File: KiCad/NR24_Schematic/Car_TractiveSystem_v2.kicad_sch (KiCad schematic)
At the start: 11 parts, among them J1 M_con, J2 F_con, K2 Key Switch Relay, M1 Zero_7R_Motor, SW3 100V E-stop (Right), SW4 100V E-stop (Left), U1 Sevcon_Gen4_Size6, U2 Throttle

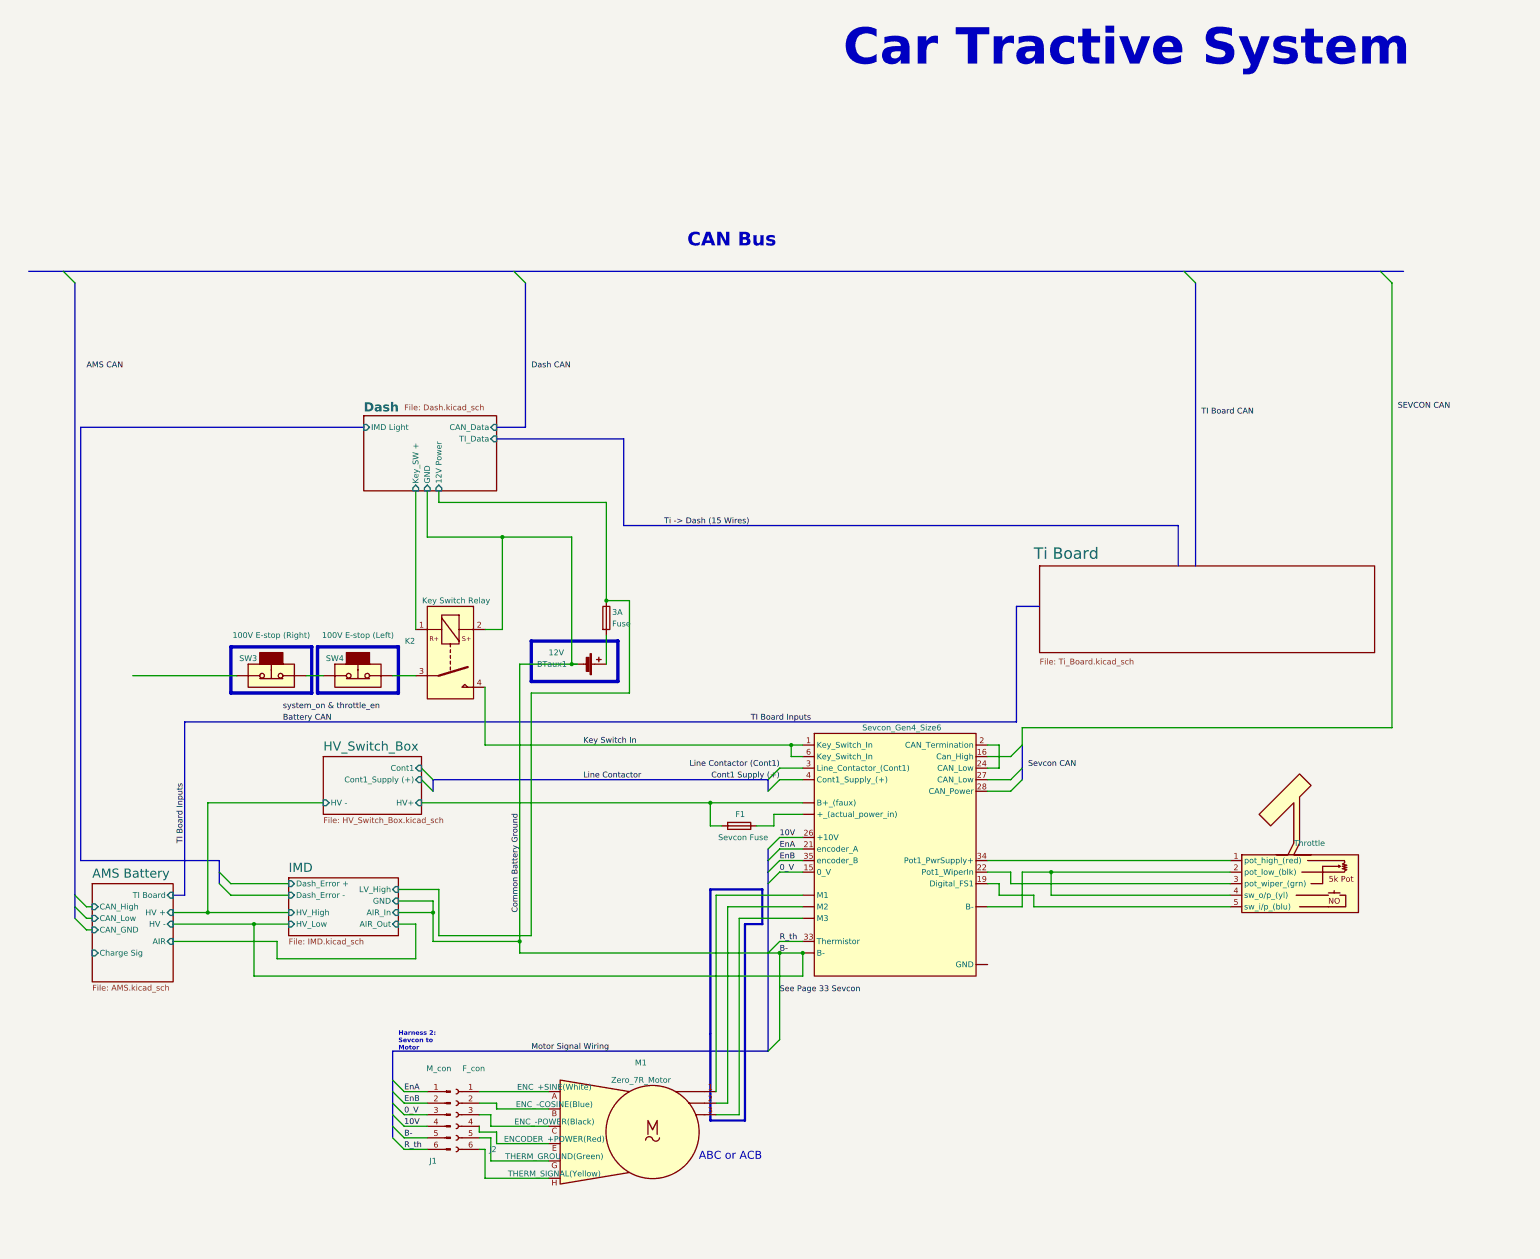
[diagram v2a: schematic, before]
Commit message: Updates
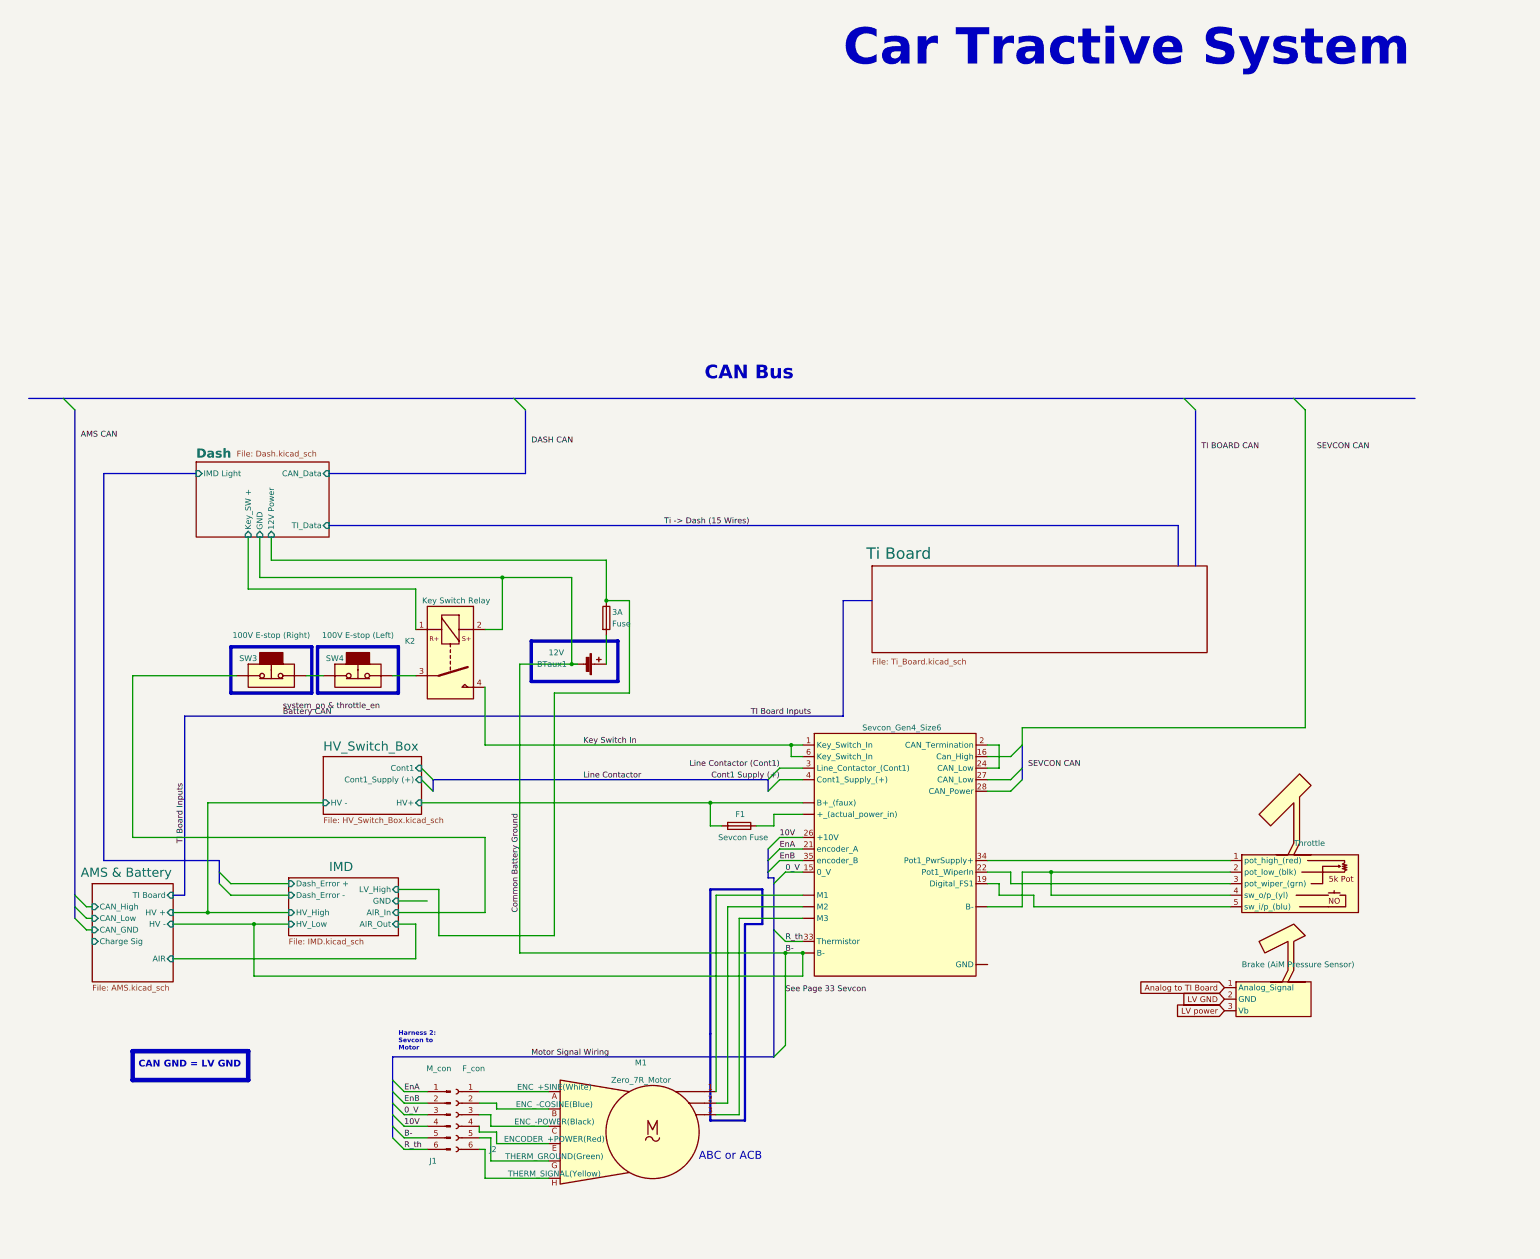
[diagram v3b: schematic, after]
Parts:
- added U7: Brake (AiM Pressure Sensor), symbol CamachosSymbols:Throttle
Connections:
- net IMD/AIR_In: now reaches SW3.1 (A)
- new net  LV power: U7.3 (Vb)
- new net Analog to TI Board: U7.1 (Analog_Signal)
- new net LV GND: U7.2 (GND)
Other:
- sheet AMS Battery renamed AMS & Battery
- note added: "CAN GND = LV GND"

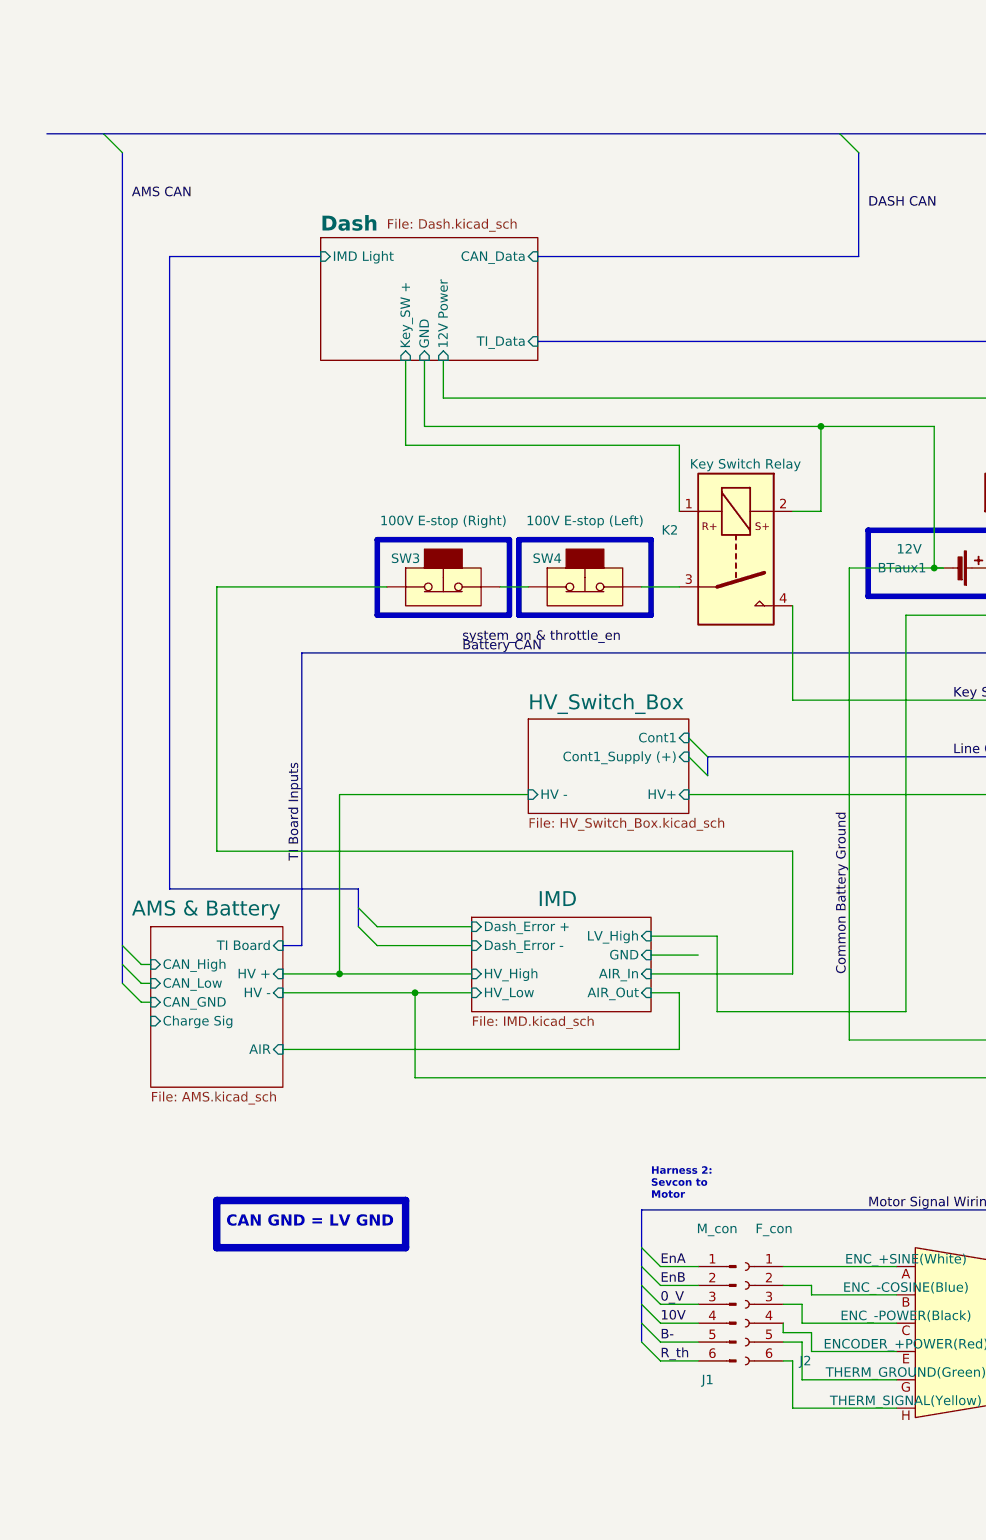
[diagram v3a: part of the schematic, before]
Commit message: Root Update
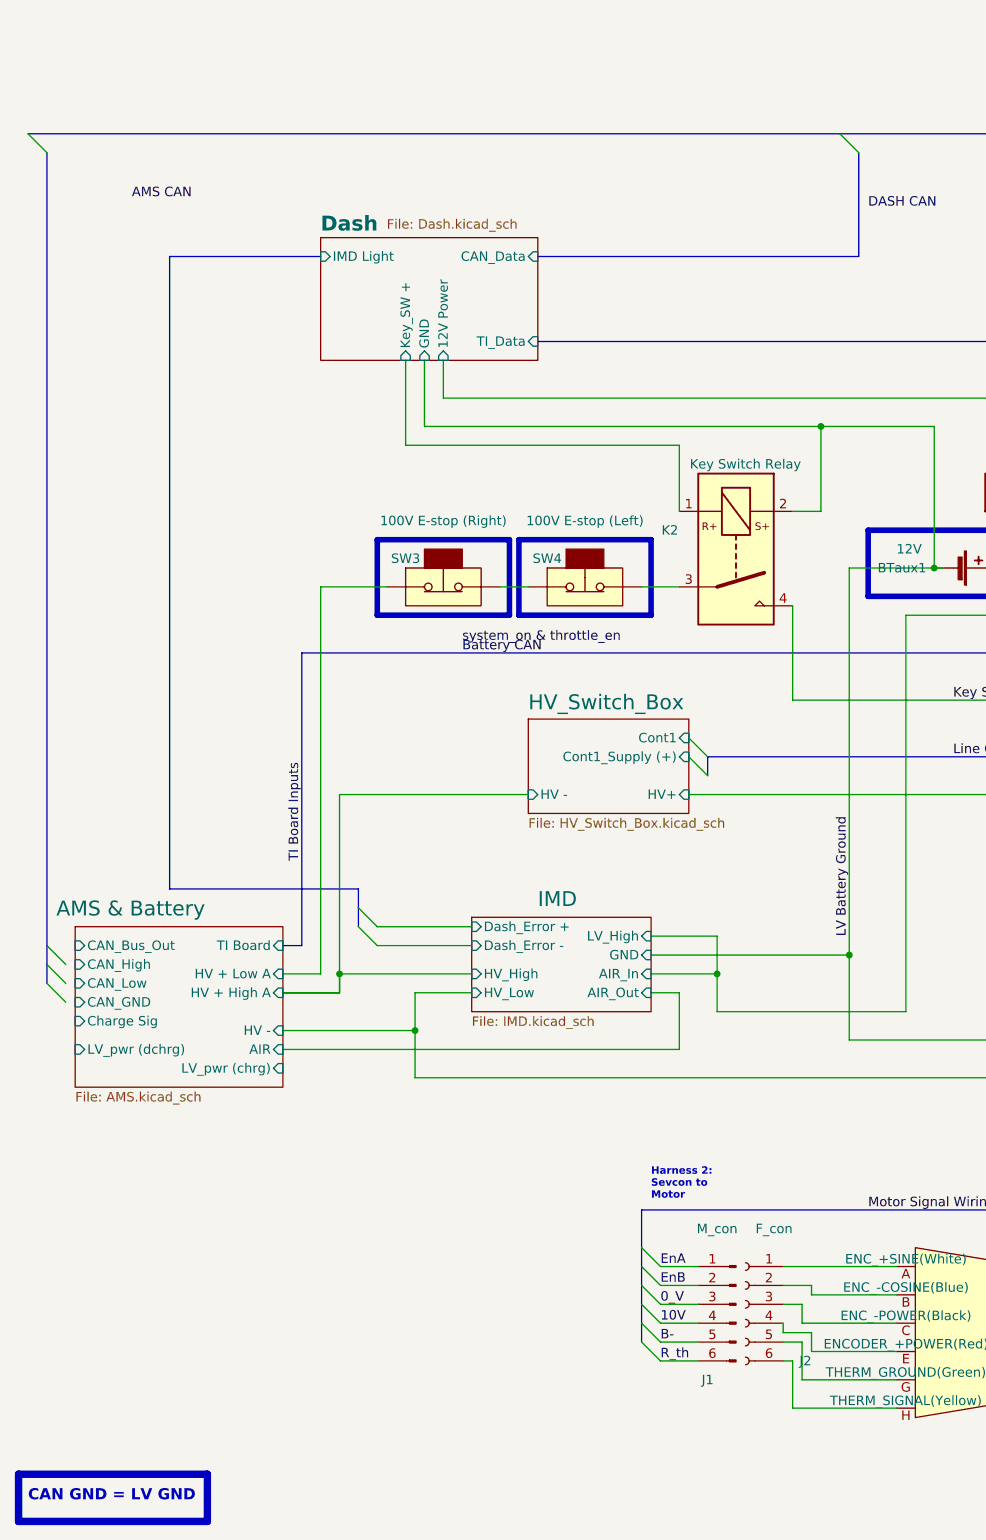
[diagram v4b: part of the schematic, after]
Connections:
- net IMD/AIR_In renamed AMS & Battery/HV + Low A
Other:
- sheet AMS & Battery ports: added CAN_Bus_Out, HV + High A, HV + Low A, LV_pwr (chrg), LV_pwr (dchrg); removed HV +
